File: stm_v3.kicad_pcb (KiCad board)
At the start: 4 copper layers, 50 x 37.8 mm, 63 parts, among them J1 OLED, J2 SWD, J3 OBDII, Q1 s8050, Q2 s8050, SW1 RST, SW2 BOOT0, SW3 LCD, SW4 MENU, U1 STM32L431RCTx, U2 SN65HVD231, U3 TPS562201, Y1 16 MHz

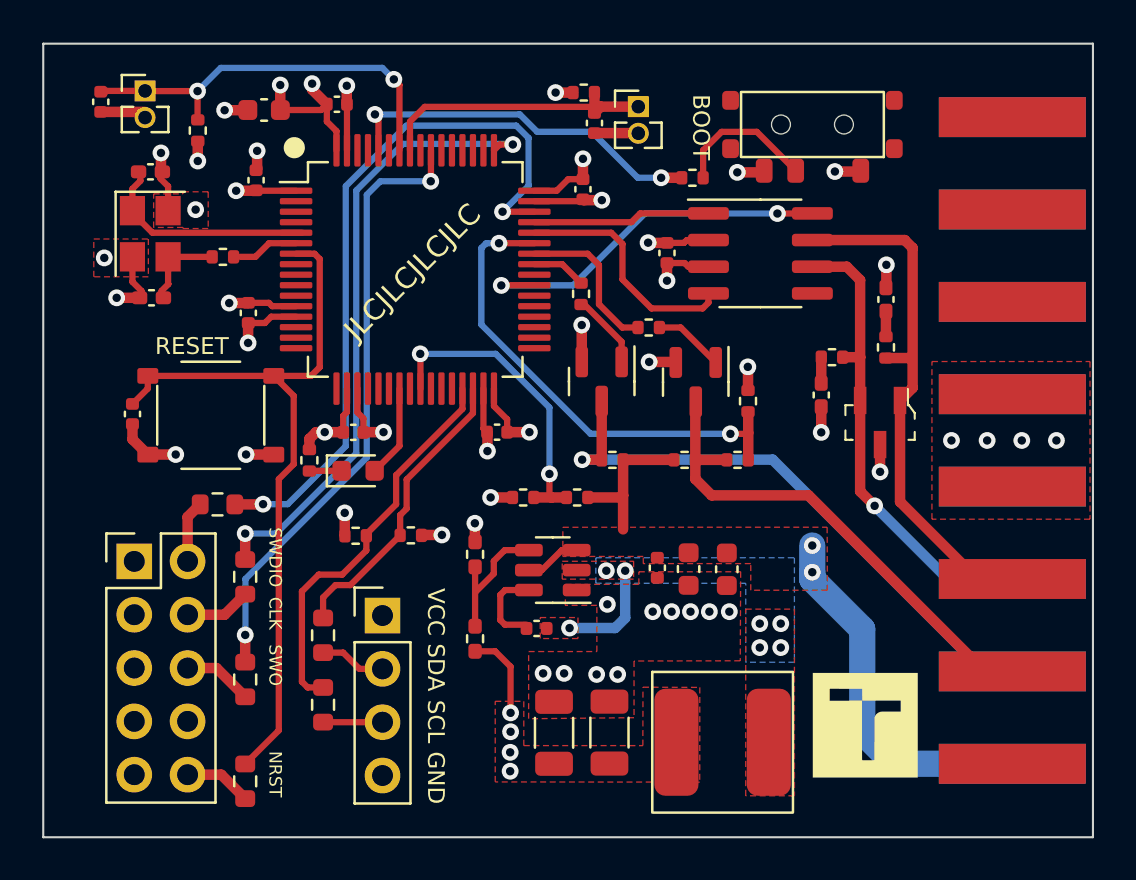
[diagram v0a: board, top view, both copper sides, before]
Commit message: Final board version
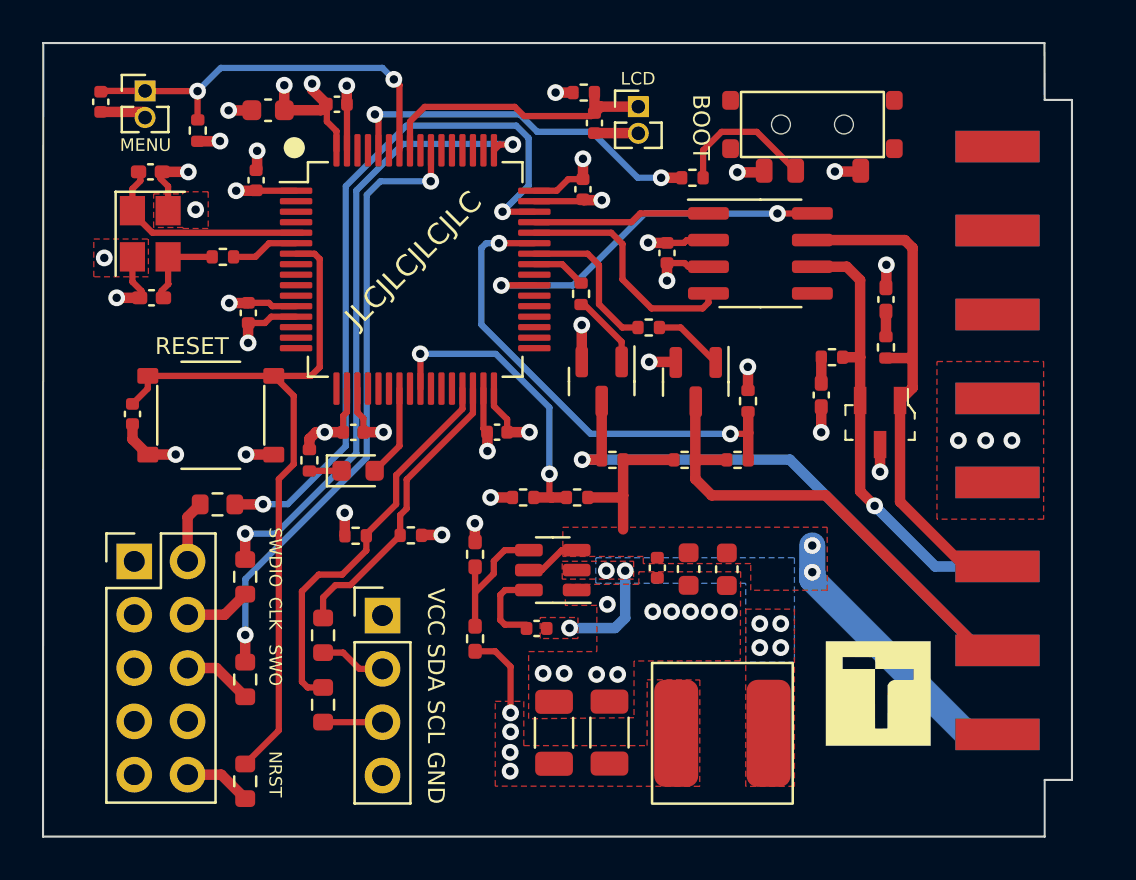
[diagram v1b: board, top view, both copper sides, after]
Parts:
- moved G*** 1.63 mm to (175.4, 98.3)
- moved J3 0.71 mm to (181.1, 86.3)
- moved L1 0.43 mm to (167.9, 100.2)
- moved C1 0.19 mm to (146.3, 70.6)
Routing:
- net +12V: track 27.8 -> 24.3 mm
- net GND: track 47.6 -> 48.0 mm, vias 37 -> 36
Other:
- board size 50 x 37.8 mm -> 49 x 37.8 mm
- board text added: "LCD"
- board text added: "MENU"
